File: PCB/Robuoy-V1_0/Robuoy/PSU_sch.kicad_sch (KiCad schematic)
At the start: 43 parts, among them J1 Accu/ESC_on-off, J5 TO FRONT SWITCH, Q1 MMBT2222A, Q2 MMBT2222A, Q201 NCE01P30K, Q3 MMBT2222A, U1 LM2595S-5, U202 AMS1117-3.3

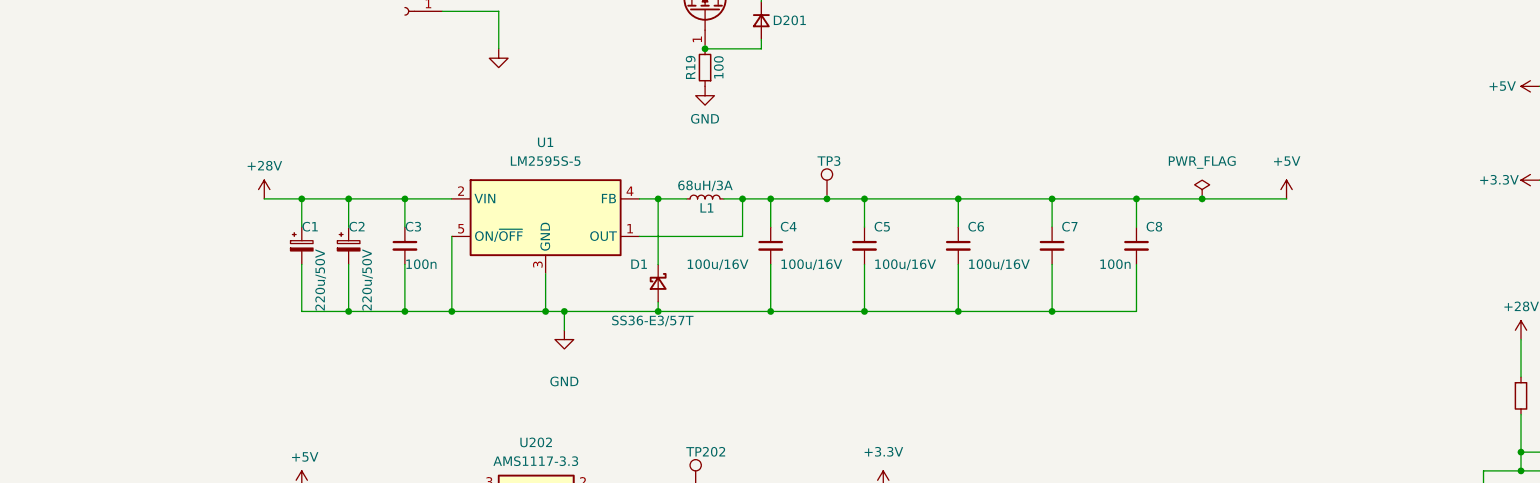
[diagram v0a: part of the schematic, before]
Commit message: auto calibrate
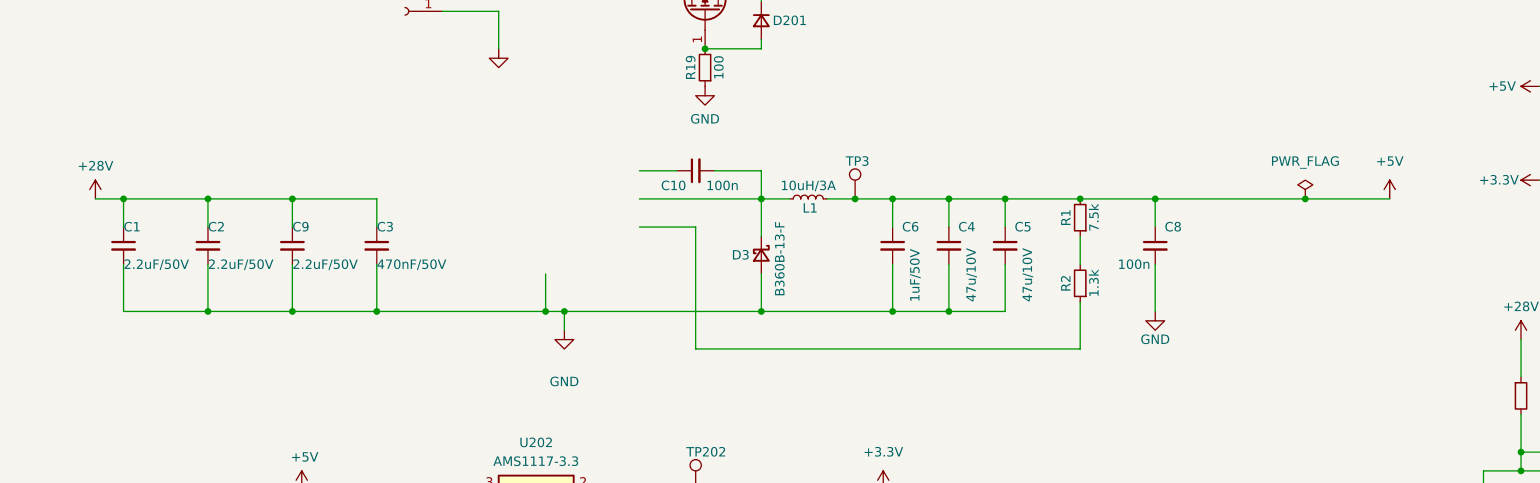
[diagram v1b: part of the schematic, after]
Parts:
- removed C1, C2: 220u/50V, A_Device:CP_ALU_D10x10.5, symbol Device:C_Polarized_Small
- removed C7: 100u/16V, Capacitor_SMD:C_1210_3225Metric, symbol Device:C_Small
- removed D1: SS36-E3/57T, A_Device:D_SMC_7.1x6.2x2.65, symbol Device:D_Schottky_Small
- removed U1: LM2595S-5, Package_TO_SOT_SMD:TO-263-5_TabPin3, symbol Regulator_Switching:LM2595S-5
- added C1, C2, C9: 2.2uF/50V, A_Device:C_0603, symbol Device:C_Small
- added C10: 100n, A_Device:C_0603, symbol Device:C_Small
- added D3: B360B-13-F, Diode_SMD:D_SMB, symbol Device:D_Schottky_Small
- added R1: 7.5k, A_Device:R_0603, symbol Device:R_Small
- added R2: 1.3k, A_Device:R_0603, symbol Device:R_Small
- C3: value 100n -> 470nF/50V; LCSC C14663 -> C513651
- C4, C5: value 100u/16V -> 47u/10V; footprint Capacitor_SMD:C_1210_3225Metric -> Capacitor_SMD:C_1206_3216Metric; LCSC C90143 -> C96123
- C6: value 100u/16V -> 1uF/50V; footprint Capacitor_SMD:C_1210_3225Metric -> Capacitor_SMD:C_0603_1608Metric; LCSC C90143 -> C1584
- L1: value 68uH/3A -> 10uH/3A; footprint A_Device:L_11.5x10.0mm -> Inductor_SMD:L_Neosid_Air-Coil_SML_6-10turn_HAM0631A-HAM1031A; LCSC C497902 -> C408412
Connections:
- net +28V: now also C1.1, C2.1, C9.1
- net +5V: now also R1.2
- net GND: now also C1.2, C2.2, C9.2, D3.2 (A)
- net at L1.1: now also C10.2, D3.1 (K)
- new net: R1.1, R2.2
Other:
- moved on the sheet: C3, C4, C8, L1, TP3
